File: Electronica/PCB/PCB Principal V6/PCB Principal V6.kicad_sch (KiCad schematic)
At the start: 19 parts, among them J1 Conexion Sensores, J12 TP, J2 Power Monster, J3 On/Off General, J4 Power Input 2, J5 IDC Placa Botones, J6 Power Input 1, J7 Conn_01x01_Pin, J8 Conn_01x01_Pin, SW1 On/Off Motores

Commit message: ,
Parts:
- LM1: footprint Step Down:LM2596_correctedMeas -> StepDown:StepDown
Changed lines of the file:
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@@
 		)
 		(instances
-			(project "PCB Principal V5"
+			(project "PCB Principal V6"
 				(path "/feeeb2cb-e374-40f4-b9c7-40ed321ecf02"
 					(reference "#PWR022")
@@
 		)
 		(instances
-			(project "PCB Principal V5"
+			(project "PCB Principal V6"
 				(path "/feeeb2cb-e374-40f4-b9c7-40ed321ecf02"
 					(reference "#PWR021")
@@
 		)
 		(instances
-			(project "PCB Principal V5"
+			(project "PCB Principal V6"
 				(path "/feeeb2cb-e374-40f4-b9c7-40ed321ecf02"
 					(reference "#PWR01")
@@
 		)
 		(instances
-			(project "PCB Principal V5"
+			(project "PCB Principal V6"
 				(path "/feeeb2cb-e374-40f4-b9c7-40ed321ecf02"
 					(reference "#PWR013")
@@
 		)
 		(instances
-			(project "PCB Principal V5"
+			(project "PCB Principal V6"
 				(path "/feeeb2cb-e374-40f4-b9c7-40ed321ecf02"
 					(reference "#PWR012")
@@
 		)
 		(instances
-			(project "PCB Principal V5"
+			(project "PCB Principal V6"
 				(path "/feeeb2cb-e374-40f4-b9c7-40ed321ecf02"
 					(reference "#PWR05")
@@
 		)
 		(instances
-			(project "PCB Principal V5"
+			(project "PCB Principal V6"
 				(path "/feeeb2cb-e374-40f4-b9c7-40ed321ecf02"
 					(reference "J1")
@@
 		)
 		(instances
-			(project "PCB Principal V5"
+			(project "PCB Principal V6"
 				(path "/feeeb2cb-e374-40f4-b9c7-40ed321ecf02"
 					(reference "D1")
@@
 		)
 		(instances
-			(project "PCB Principal V5"
+			(project "PCB Principal V6"
 				(path "/feeeb2cb-e374-40f4-b9c7-40ed321ecf02"
 					(reference "#PWR019")
@@
 		)
 		(instances
-			(project "PCB Principal V5"
+			(project "PCB Principal V6"
 				(path "/feeeb2cb-e374-40f4-b9c7-40ed321ecf02"
 					(reference "J5")
@@
 		)
 		(instances
-			(project "PCB Principal V5"
+			(project "PCB Principal V6"
 				(path "/feeeb2cb-e374-40f4-b9c7-40ed321ecf02"
 					(reference "J3")
@@
 		)
 		(instances
-			(project "PCB Principal V5"
+			(project "PCB Principal V6"
 				(path "/feeeb2cb-e374-40f4-b9c7-40ed321ecf02"
 					(reference "#PWR017")
@@
 		)
 		(instances
-			(project "PCB Principal V5"
+			(project "PCB Principal V6"
 				(path "/feeeb2cb-e374-40f4-b9c7-40ed321ecf02"
 					(reference "#PWR07")
@@
 		)
 		(instances
-			(project "PCB Principal V5"
+			(project "PCB Principal V6"
 				(path "/feeeb2cb-e374-40f4-b9c7-40ed321ecf02"
 					(reference "D4")
@@
 			)
 		)
-		(property "Footprint" "Step Down:LM2596_correctedMeas"
+		(property "Footprint" "StepDown:StepDown"
 			(at 119.38 123.19 0)
 			(effects
@@
 		)
 		(instances
-			(project "PCB Principal V5"
+			(project "PCB Principal V6"
 				(path "/feeeb2cb-e374-40f4-b9c7-40ed321ecf02"
 					(reference "LM1")
@@
 		)
 		(instances
-			(project "PCB Principal V5"
+			(project "PCB Principal V6"
 				(path "/feeeb2cb-e374-40f4-b9c7-40ed321ecf02"
 					(reference "SW1")
@@
 		)
 		(instances
-			(project "PCB Principal V5"
+			(project "PCB Principal V6"
 				(path "/feeeb2cb-e374-40f4-b9c7-40ed321ecf02"
 					(reference "#PWR02")
@@
 		)
 		(instances
-			(project "PCB Principal V5"
+			(project "PCB Principal V6"
 				(path "/feeeb2cb-e374-40f4-b9c7-40ed321ecf02"
 					(reference "#PWR015")
@@
 		)
 		(instances
-			(project "PCB Principal V5"
+			(project "PCB Principal V6"
 				(path "/feeeb2cb-e374-40f4-b9c7-40ed321ecf02"
 					(reference "D2")
@@
 		)
 		(instances
-			(project "PCB Principal V5"
+			(project "PCB Principal V6"
 				(path "/feeeb2cb-e374-40f4-b9c7-40ed321ecf02"
 					(reference "R2")
@@
 		)
 		(instances
-			(project "PCB Principal V5"
+			(project "PCB Principal V6"
 				(path "/feeeb2cb-e374-40f4-b9c7-40ed321ecf02"
 					(reference "J7")
@@
 		)
 		(instances
-			(project "PCB Principal V5"
+			(project "PCB Principal V6"
 				(path "/feeeb2cb-e374-40f4-b9c7-40ed321ecf02"
 					(reference "#PWR011")
@@
 		)
 		(instances
-			(project "PCB Principal V5"
+			(project "PCB Principal V6"
 				(path "/feeeb2cb-e374-40f4-b9c7-40ed321ecf02"
 					(reference "D3")
@@
 		)
 		(instances
-			(project "PCB Principal V5"
+			(project "PCB Principal V6"
 				(path "/feeeb2cb-e374-40f4-b9c7-40ed321ecf02"
 					(reference "#PWR08")
@@
 		)
 		(instances
-			(project "PCB Principal V5"
+			(project "PCB Principal V6"
 				(path "/feeeb2cb-e374-40f4-b9c7-40ed321ecf02"
 					(reference "#PWR016")
@@
 		)
 		(instances
-			(project "PCB Principal V5"
+			(project "PCB Principal V6"
 				(path "/feeeb2cb-e374-40f4-b9c7-40ed321ecf02"
 					(reference "#PWR020")
@@
 		)
 		(instances
-			(project "PCB Principal V5"
+			(project "PCB Principal V6"
 				(path "/feeeb2cb-e374-40f4-b9c7-40ed321ecf02"
 					(reference "R1")
@@
 		)
 		(instances
-			(project "PCB Principal V5"
+			(project "PCB Principal V6"
 				(path "/feeeb2cb-e374-40f4-b9c7-40ed321ecf02"
 					(reference "J6")
@@
 		)
 		(instances
-			(project "PCB Principal V5"
+			(project "PCB Principal V6"
 				(path "/feeeb2cb-e374-40f4-b9c7-40ed321ecf02"
 					(reference "#PWR04")
@@
 		)
 		(instances
-			(project "PCB Principal V5"
+			(project "PCB Principal V6"
 				(path "/feeeb2cb-e374-40f4-b9c7-40ed321ecf02"
 					(reference "#PWR03")
@@
 		)
 		(instances
-			(project "PCB Principal V5"
+			(project "PCB Principal V6"
 				(path "/feeeb2cb-e374-40f4-b9c7-40ed321ecf02"
 					(reference "J2")
@@
 		)
 		(instances
-			(project "PCB Principal V5"
+			(project "PCB Principal V6"
 				(path "/feeeb2cb-e374-40f4-b9c7-40ed321ecf02"
 					(reference "J8")
@@
 		)
 		(instances
-			(project "PCB Principal V5"
+			(project "PCB Principal V6"
 				(path "/feeeb2cb-e374-40f4-b9c7-40ed321ecf02"
 					(reference "#PWR09")
@@
 		)
 		(instances
-			(project "PCB Principal V5"
+			(project "PCB Principal V6"
 				(path "/feeeb2cb-e374-40f4-b9c7-40ed321ecf02"
 					(reference "J4")
@@
 		)
 		(instances
-			(project "PCB Principal V5"
+			(project "PCB Principal V6"
 				(path "/feeeb2cb-e374-40f4-b9c7-40ed321ecf02"
 					(reference "A1")
@@
 		)
 		(instances
-			(project "PCB Principal V5"
+			(project "PCB Principal V6"
 				(path "/feeeb2cb-e374-40f4-b9c7-40ed321ecf02"
 					(reference "J12")
@@
 		)
 		(instances
-			(project "PCB Principal V5"
+			(project "PCB Principal V6"
 				(path "/feeeb2cb-e374-40f4-b9c7-40ed321ecf02"
 					(reference "#PWR010")
@@
 		)
 		(instances
-			(project "PCB Principal V5"
+			(project "PCB Principal V6"
 				(path "/feeeb2cb-e374-40f4-b9c7-40ed321ecf02"
 					(reference "A2")
@@
 		)
 		(instances
-			(project "PCB Principal V5"
+			(project "PCB Principal V6"
 				(path "/feeeb2cb-e374-40f4-b9c7-40ed321ecf02"
 					(reference "#PWR014")
@@
 		)
 		(instances
-			(project "PCB Principal V5"
+			(project "PCB Principal V6"
 				(path "/feeeb2cb-e374-40f4-b9c7-40ed321ecf02"
 					(reference "#PWR018")
@@
 		)
 		(instances
-			(project "PCB Principal V5"
+			(project "PCB Principal V6"
 				(path "/feeeb2cb-e374-40f4-b9c7-40ed321ecf02"
 					(reference "#PWR06")

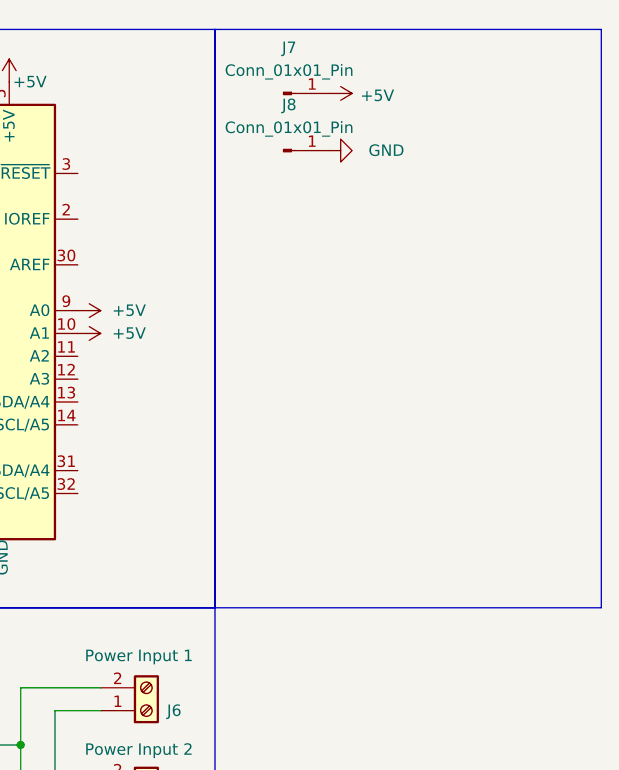
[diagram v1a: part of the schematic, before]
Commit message: PCB CHERNIAK TERMINAR
TONTO EL QUE LEE
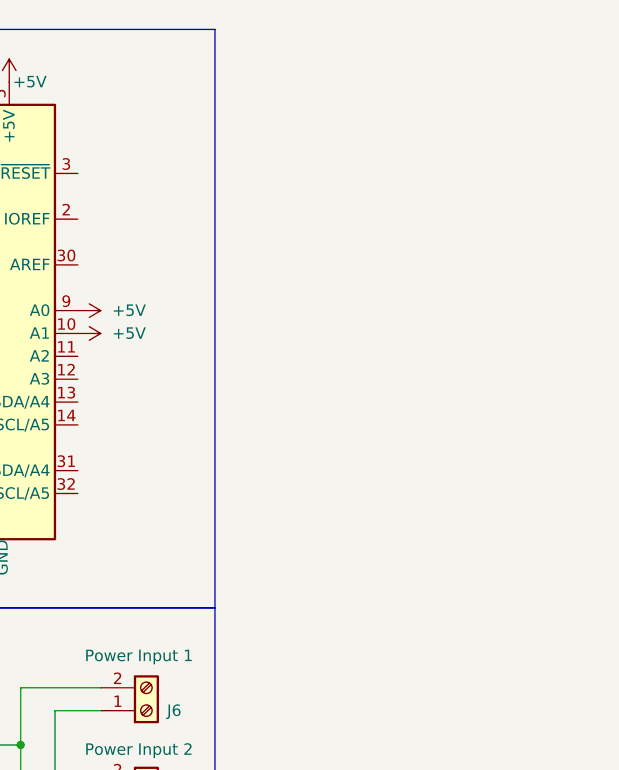
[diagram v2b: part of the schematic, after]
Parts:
- removed J7, J8: Conn_01x01_Pin, Connector_PinHeader_2.54mm:PinHeader_1x01_P2.54mm_Vertical, symbol Connector:Conn_01x01_Pin

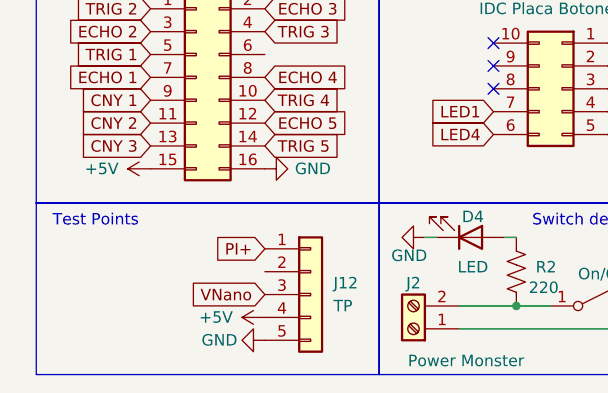
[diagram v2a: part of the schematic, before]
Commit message: pcb terminar?
TONTO EL QUE LEE
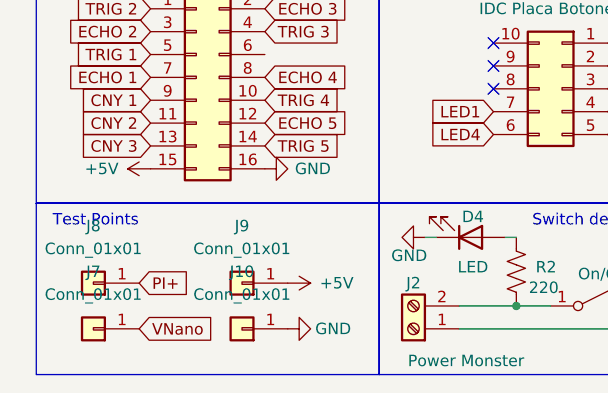
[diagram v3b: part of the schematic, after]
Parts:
- removed J12: TP, Connector_PinHeader_2.54mm:PinHeader_1x05_P2.54mm_Vertical, symbol Connector_Generic:Conn_01x05
- added J10, J7, J8, J9: Conn_01x01, Connector_PinHeader_2.54mm:PinHeader_1x01_P2.54mm_Vertical, symbol Connector_Generic:Conn_01x01
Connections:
- net +5V: now also J9.1 (Pin_1)
- net GND: now also J10.1 (Pin_1)
- net PI+: now also J8.1 (Pin_1)
- net VNano: now also J7.1 (Pin_1)

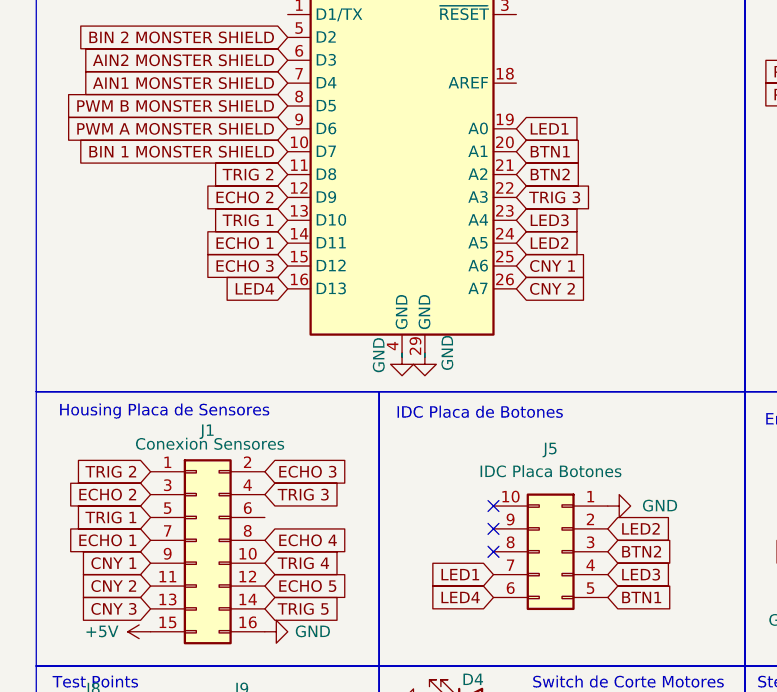
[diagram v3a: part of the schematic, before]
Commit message: .
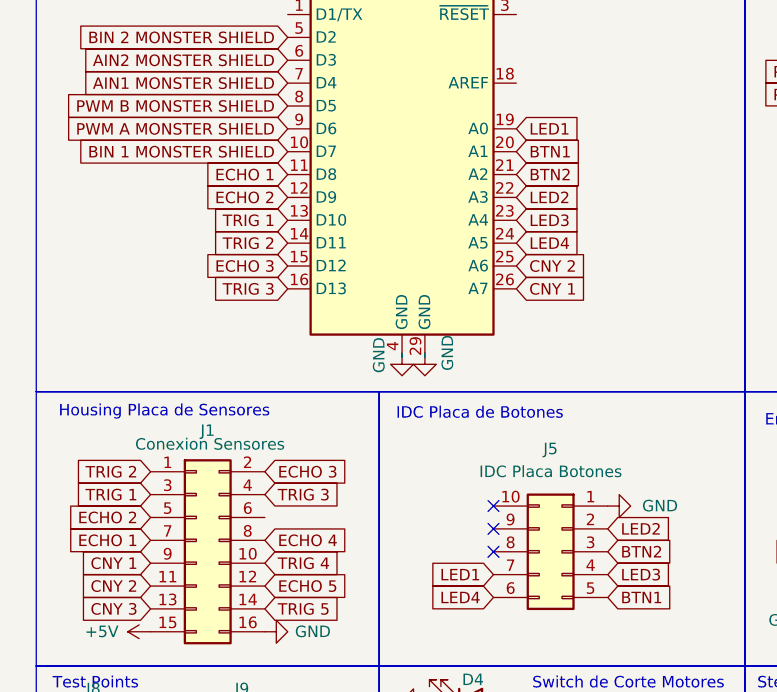
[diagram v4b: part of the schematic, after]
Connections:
- net CNY 1: now also A1.26 (A7); no longer A1.25 (A6)
- net CNY 2: now also A1.25 (A6); no longer A1.26 (A7)
- net ECHO 1: now also A1.11 (D8); no longer A1.14 (D11)
- net ECHO 2: now also J1.5 (Pin_5); no longer J1.3 (Pin_3)
- net LED2: now also A1.22 (A3); no longer A1.24 (A5)
- net LED4: now also A1.24 (A5); no longer A1.16 (D13)
- net TRIG 1: now also J1.3 (Pin_3); no longer J1.5 (Pin_5)
- net TRIG 2: now also A1.14 (D11); no longer A1.11 (D8)
- net TRIG 3: now also A1.16 (D13); no longer A1.22 (A3)
